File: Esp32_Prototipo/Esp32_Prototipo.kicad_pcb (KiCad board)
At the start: 2 copper layers, 100 x 85 mm, 18 parts, among them J1 Fan, J2 Screw_Terminal_01x04, J3 Screw_Terminal_01x04, J4 Input, Q1 2N7002K, U1 ESP32-DEVKITC-32D

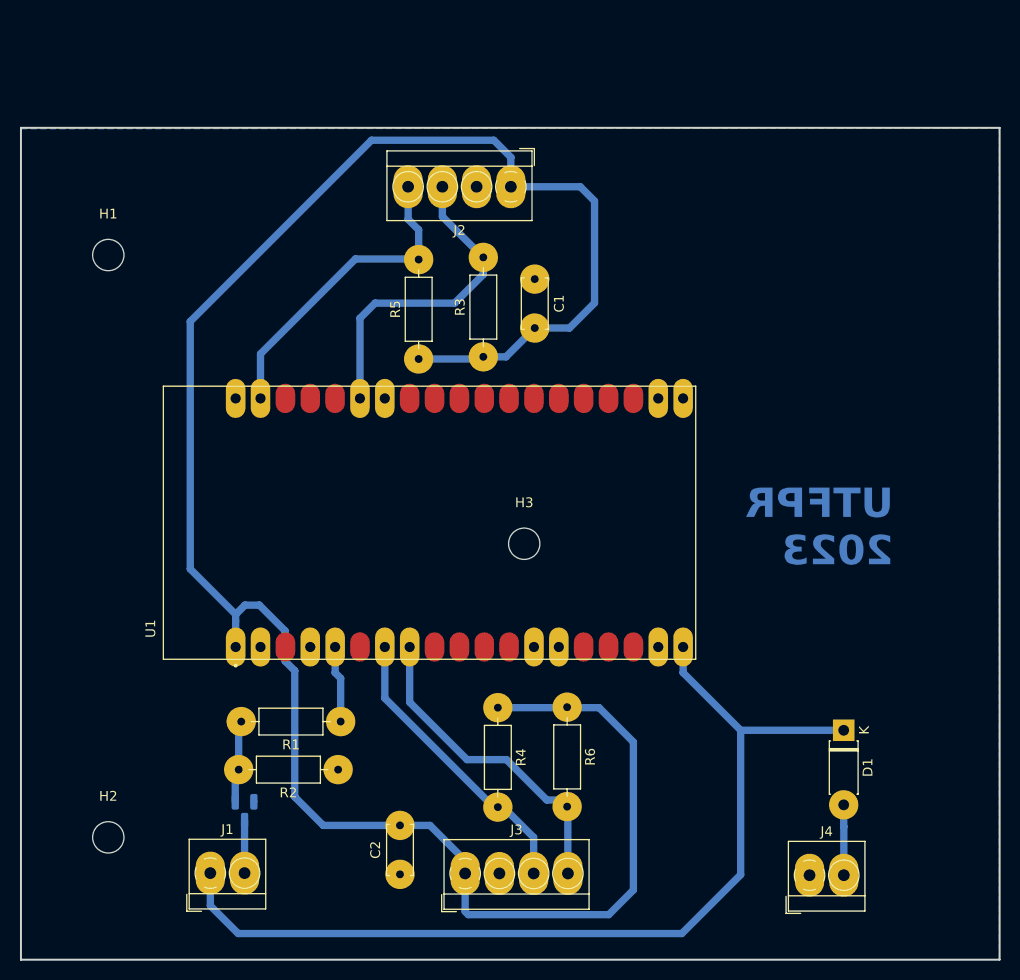
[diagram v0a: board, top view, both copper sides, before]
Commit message: proto esp32 pronto para montar
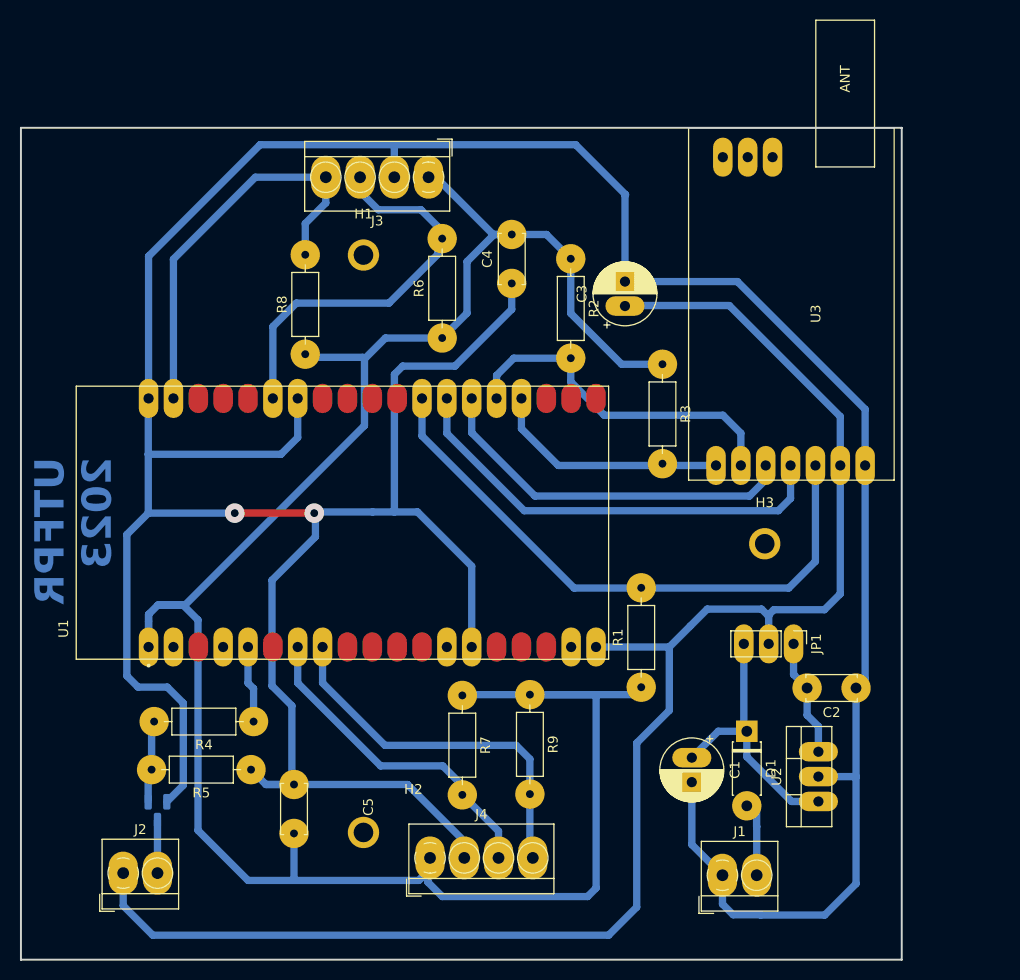
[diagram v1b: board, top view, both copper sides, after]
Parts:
- added C1: 100uF, Capacitor_THT:CP_Radial_D6.3mm_P2.50mm, F.Cu at (164.4, 112.7)
- added C2: 220n, Capacitor_THT:C_Disc_D5.0mm_W2.5mm_P5.00mm, F.Cu at (181.2, 105.5)
- added C3: 100uF, Capacitor_THT:CP_Radial_D6.3mm_P2.50mm, F.Cu at (157.6, 66.5)
- added JP1: Jumper_3_Bridged12, Connector_PinHeader_2.54mm:PinHeader_1x03_P2.54mm_Vertical, F.Cu at (174.8, 101.0)
- added R1: 2k2, Resistor_THT:R_Axial_DIN0207_L6.3mm_D2.5mm_P10.16mm_Horizontal, F.Cu at (159.3, 105.5)
- added R2: 2k2, Resistor_THT:R_Axial_DIN0207_L6.3mm_D2.5mm_P10.16mm_Horizontal, F.Cu at (152.1, 61.7)
- added R3: 2k2, Resistor_THT:R_Axial_DIN0207_L6.3mm_D2.5mm_P10.16mm_Horizontal, F.Cu at (161.4, 72.5)
- added U2: LM7805_TO220, Package_TO_SOT_THT:TO-220-3_Vertical, F.Cu at (177.4, 117.1)
- added U3: E32-433T20D, footprints6:E32-xxxT20D, F.Cu at (164.1, 84.3)
- moved H2 26.1 mm to (130.9, 120.3)
- moved H1 26.1 mm to (130.9, 61.3)
- moved H3 24.6 mm to (171.9, 90.8)
- moved C5 14.2 mm to (123.8, 115.4), turned to -90 degrees
- moved R8 11.6 mm to (124.9, 71.4)
- moved D1 9.90 mm to (170.1, 110.0)
- moved J1 8.90 mm to (167.6, 124.7)
- moved J2 8.90 mm to (106.3, 124.5)
- moved Q1 8.90 mm to (109.8, 118.1)
- moved R5 8.90 mm to (119.4, 113.9)
- moved U1 8.90 mm to (128.7, 88.7)
- moved R4 8.90 mm to (119.7, 109.0)
- moved J3 8.47 mm to (137.5, 53.4)
- moved R6 4.62 mm to (138.9, 69.8)
- moved R9 4.02 mm to (147.9, 106.2)
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- renumbered C1 to C4, C2 to C5, J4 to J1, J1 to J2, J2 to J3, J3 to J4, R1 to R4, R2 to R5, R3 to R6, R4 to R7, R5 to R8, R6 to R9
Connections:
- D1 pad 1: +BATT -> Net-(D1-K)
- U1 pad J3-12: unconnected-(U1-IO16-PadJ3-12) -> AUX
- U1 pad J3-13: unconnected-(U1-IO4-PadJ3-13) -> TXD
- U1 pad J3-14: unconnected-(U1-IO0-PadJ3-14) -> RXD
- U1 pad J3-15: unconnected-(U1-IO2-PadJ3-15) -> M1
- U1 pad J3-16: unconnected-(U1-IO15-PadJ3-16) -> M0
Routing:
- net GND: track 0.00 -> 396.8 mm, vias 0 -> 2
- net +BATT: track 97.4 -> 161.7 mm
- net AUX: track 0.00 -> 61.4 mm
- net TXD: track 0.00 -> 45.9 mm
- net RXD: track 0.00 -> 38.4 mm
- net M1: track 0.00 -> 35.9 mm
- net Net-(D1-K): track 0.00 -> 27.6 mm
- net M0: track 0.00 -> 24.5 mm
- net +3V3: track 217.3 -> 231.9 mm
- net Net-(JP1-A): track 0.00 -> 12.1 mm
- net SDA0: track 32.6 -> 42.7 mm
- net SCL0: track 33.3 -> 40.2 mm
- net SCL1: track 30.0 -> 35.4 mm
- net SDA1: track 33.0 -> 38.3 mm
- removed copper zone on B.Cu, net GND
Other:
- board size 100 x 85 mm -> 90 x 85 mm
